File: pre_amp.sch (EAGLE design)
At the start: 51 parts, among them Q1 BF245, Q2 BF245, Q3 BF245

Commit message: [#1] Update component package
Update component package.
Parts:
- C4: device rcl:C-US375-203X418 -> rcl:C-US050-030X075
- C8: device rcl:C-US375-203X418 -> rcl:C-US050-025X075
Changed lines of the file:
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@@
 <grid distance="0.1" unitdist="inch" unit="inch" style="dots" multiple="1" display="yes" altdistance="0.01" altunitdist="inch" altunit="inch"/>
 <layers>
-<layer number="1" name="Top" color="4" fill="1" visible="no" active="no"/>
-<layer number="16" name="Bottom" color="1" fill="1" visible="no" active="no"/>
-<layer number="17" name="Pads" color="2" fill="1" visible="no" active="no"/>
-<layer number="18" name="Vias" color="2" fill="1" visible="no" active="no"/>
-<layer number="19" name="Unrouted" color="6" fill="1" visible="no" active="no"/>
-<layer number="20" name="Dimension" color="15" fill="1" visible="no" active="no"/>
-<layer number="21" name="tPlace" color="7" fill="1" visible="no" active="no"/>
-<layer number="22" name="bPlace" color="7" fill="1" visible="no" active="no"/>
-<layer number="23" name="tOrigins" color="15" fill="1" visible="no" active="no"/>
-<layer number="24" name="bOrigins" color="15" fill="1" visible="no" active="no"/>
-<layer number="25" name="tNames" color="7" fill="1" visible="no" active="no"/>
-<layer number="26" name="bNames" color="7" fill="1" visible="no" active="no"/>
-<layer number="27" name="tValues" color="7" fill="1" visible="no" active="no"/>
-<layer number="28" name="bValues" color="7" fill="1" visible="no" active="no"/>
+<layer number="1" name="Top" color="4" fill="1" visible="yes" active="no"/>
+<layer number="16" name="Bottom" color="1" fill="1" visible="yes" active="no"/>
+<layer number="17" name="Pads" color="2" fill="1" visible="yes" active="no"/>
+<layer number="18" name="Vias" color="2" fill="1" visible="yes" active="no"/>
+<layer number="19" name="Unrouted" color="6" fill="1" visible="yes" active="no"/>
+<layer number="20" name="Dimension" color="15" fill="1" visible="yes" active="no"/>
+<layer number="21" name="tPlace" color="7" fill="1" visible="yes" active="no"/>
+<layer number="22" name="bPlace" color="7" fill="1" visible="yes" active="no"/>
+<layer number="23" name="tOrigins" color="15" fill="1" visible="yes" active="no"/>
+<layer number="24" name="bOrigins" color="15" fill="1" visible="yes" active="no"/>
+<layer number="25" name="tNames" color="7" fill="1" visible="yes" active="no"/>
+<layer number="26" name="bNames" color="7" fill="1" visible="yes" active="no"/>
+<layer number="27" name="tValues" color="7" fill="1" visible="yes" active="no"/>
+<layer number="28" name="bValues" color="7" fill="1" visible="yes" active="no"/>
 <layer number="29" name="tStop" color="7" fill="3" visible="no" active="no"/>
 <layer number="30" name="bStop" color="7" fill="6" visible="no" active="no"/>
@@
 <layer number="35" name="tGlue" color="7" fill="4" visible="no" active="no"/>
 <layer number="36" name="bGlue" color="7" fill="5" visible="no" active="no"/>
-<layer number="37" name="tTest" color="7" fill="1" visible="no" active="no"/>
-<layer number="38" name="bTest" color="7" fill="1" visible="no" active="no"/>
+<layer number="37" name="tTest" color="7" fill="1" visible="yes" active="no"/>
+<layer number="38" name="bTest" color="7" fill="1" visible="yes" active="no"/>
 <layer number="39" name="tKeepout" color="4" fill="11" visible="no" active="no"/>
 <layer number="40" name="bKeepout" color="1" fill="11" visible="no" active="no"/>
@@
 <layer number="44" name="Drills" color="7" fill="1" visible="no" active="no"/>
 <layer number="45" name="Holes" color="7" fill="1" visible="no" active="no"/>
-<layer number="46" name="Milling" color="3" fill="1" visible="no" active="no"/>
-<layer number="47" name="Measures" color="7" fill="1" visible="no" active="no"/>
-<layer number="48" name="Document" color="7" fill="1" visible="no" active="no"/>
-<layer number="49" name="Reference" color="7" fill="1" visible="no" active="no"/>
-<layer number="51" name="tDocu" color="7" fill="1" visible="no" active="no"/>
-<layer number="52" name="bDocu" color="7" fill="1" visible="no" active="no"/>
+<layer number="46" name="Milling" color="3" fill="1" visible="yes" active="no"/>
+<layer number="47" name="Measures" color="7" fill="1" visible="yes" active="no"/>
+<layer number="48" name="Document" color="7" fill="1" visible="yes" active="no"/>
+<layer number="49" name="Reference" color="7" fill="1" visible="yes" active="no"/>
+<layer number="51" name="tDocu" color="7" fill="1" visible="yes" active="no"/>
+<layer number="52" name="bDocu" color="7" fill="1" visible="yes" active="no"/>
 <layer number="90" name="Modules" color="5" fill="1" visible="yes" active="yes"/>
 <layer number="91" name="Nets" color="2" fill="1" visible="yes" active="yes"/>
@@
 <part name="Q2" library="transistor-fet" deviceset="BF245" device=""/>
 <part name="Q3" library="transistor-fet" deviceset="BF245" device=""/>
-<part name="C4" library="rcl" deviceset="C-US" device="375-203X418" value="6n8"/>
+<part name="C4" library="rcl" deviceset="C-US" device="050-030X075" value="6n8"/>
 <part name="C5" library="rcl" deviceset="C-US" device="050-030X075" value="10n"/>
 <part name="LOW_IN" library="solpad" deviceset="MCS08" device=""/>
@@
 <part name="GND9" library="supply1" deviceset="GND" device=""/>
 <part name="R14" library="pot" deviceset="3RP/1610N" device="" value="1M Log - Vol"/>
-<part name="C8" library="rcl" deviceset="C-US" device="375-203X418" value="330p"/>
+<part name="C8" library="rcl" deviceset="C-US" device="050-025X075" value="330p"/>
 <part name="GND10" library="supply1" deviceset="GND" device=""/>
 <part name="ULTRA_HIGH_2" library="solpad" deviceset="MCS08" device=""/>

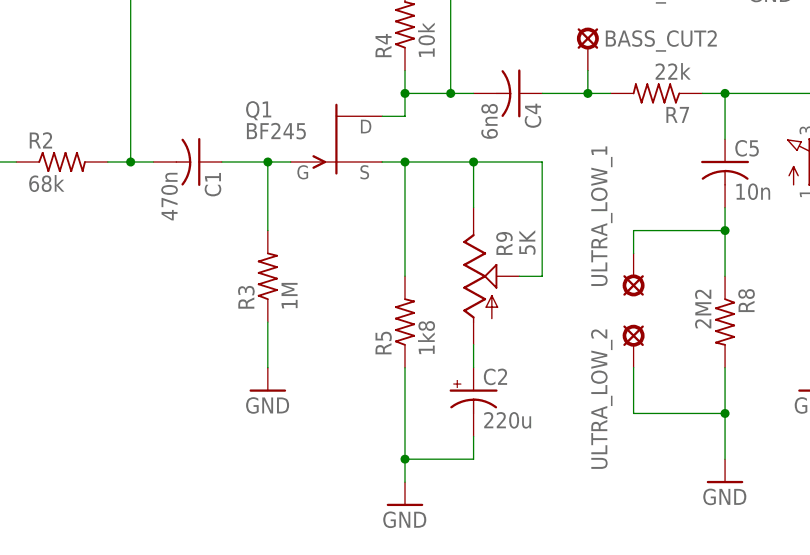
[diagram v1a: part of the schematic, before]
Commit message: [#1] PCB layout
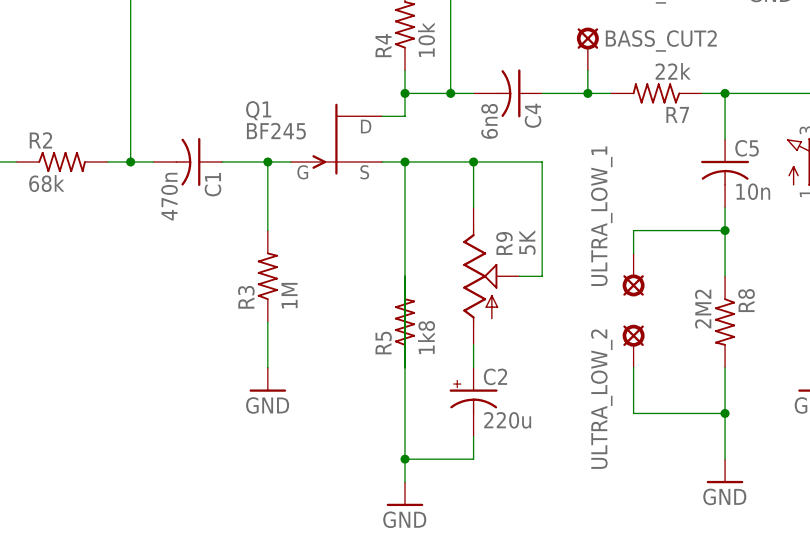
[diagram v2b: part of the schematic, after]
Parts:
- C2: device resistor:CPOL-USE3.5-8 -> resistor:CPOL-USE5-8.5
- R5: device resistor:R-US_0204/7 -> resistor:R-US_0207/10
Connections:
- net GND: now also R5.2; no longer R5.1
- net N$4: now also R5.1; no longer R5.2
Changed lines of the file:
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@@
 </variantdefs>
 <classes>
-<class number="0" name="default" width="0" drill="0">
+<class number="0" name="default" width="1.016" drill="0">
+<clearance class="0" value="0.8128"/>
+</class>
+<class number="1" name="Power" width="1.2192" drill="0">
+<clearance class="1" value="1.016"/>
 </class>
 </classes>
@@
 <part name="R3" library="resistor" deviceset="R-US_" device="0204/7" value="1M"/>
 <part name="R4" library="resistor" deviceset="R-US_" device="0204/7" value="10k"/>
-<part name="R5" library="resistor" deviceset="R-US_" device="0204/7" value="1k8"/>
+<part name="R5" library="resistor" deviceset="R-US_" device="0207/10" value="1k8"/>
 <part name="R6" library="resistor" deviceset="R-US_" device="0204/7" value="2M2"/>
 <part name="R7" library="resistor" deviceset="R-US_" device="0204/7" value="22k"/>
 <part name="R8" library="resistor" deviceset="R-US_" device="0204/7" value="2M2"/>
 <part name="C1" library="resistor" deviceset="C-US" device="050-035X075" value="470n"/>
-<part name="C2" library="resistor" deviceset="CPOL-US" device="E3.5-8" value="220u"/>
+<part name="C2" library="resistor" deviceset="CPOL-US" device="E5-8.5" value="220u"/>
 <part name="C3" library="resistor" deviceset="CPOL-US" device="E2.5-6" value="4u7"/>
 <part name="Q1" library="transistor-fet" deviceset="BF245" device=""/>
@@
 <segment>
 <pinref part="Q1" gate="G$1" pin="S"/>
-<pinref part="R5" gate="G$1" pin="2"/>
+<pinref part="R5" gate="G$1" pin="1"/>
 <wire x1="78.74" y1="71.12" x2="81.28" y2="71.12" width="0.1524" layer="91"/>
-<wire x1="81.28" y1="71.12" x2="81.28" y2="58.42" width="0.1524" layer="91"/>
+<wire x1="81.28" y1="71.12" x2="81.28" y2="48.26" width="0.1524" layer="91"/>
 <pinref part="R9" gate="G$1" pin="E"/>
 <wire x1="88.9" y1="66.04" x2="88.9" y2="71.12" width="0.1524" layer="91"/>
@@
 </segment>
 </net>
-<net name="GND" class="0">
+<net name="GND" class="1">
 <segment>
 <pinref part="HIGH_RET" gate="G$1" pin="MP"/>
@@
 </segment>
 <segment>
-<pinref part="R5" gate="G$1" pin="1"/>
-<wire x1="81.28" y1="48.26" x2="81.28" y2="38.1" width="0.1524" layer="91"/>
+<pinref part="R5" gate="G$1" pin="2"/>
+<wire x1="81.28" y1="58.42" x2="81.28" y2="38.1" width="0.1524" layer="91"/>
 <pinref part="C2" gate="G$1" pin="-"/>
 <wire x1="81.28" y1="38.1" x2="88.9" y2="38.1" width="0.1524" layer="91"/>
@@
 </segment>
 </net>
-<net name="VCC" class="0">
+<net name="VCC" class="1">
 <segment>
 <pinref part="R4" gate="G$1" pin="2"/>
